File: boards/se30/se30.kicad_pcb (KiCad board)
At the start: 2 copper layers, 116.8 x 59.7 mm, 43 parts, among them J1 Mac SE/30 PDS Interface, J2 Conn_02x05_Odd_Even, U1 ENC624J600-PT, U2 SST39SF010, U3 GAL16V8, U4 GAL16V8, U5 LD1117S33TR_SOT223, Y1 25MHz

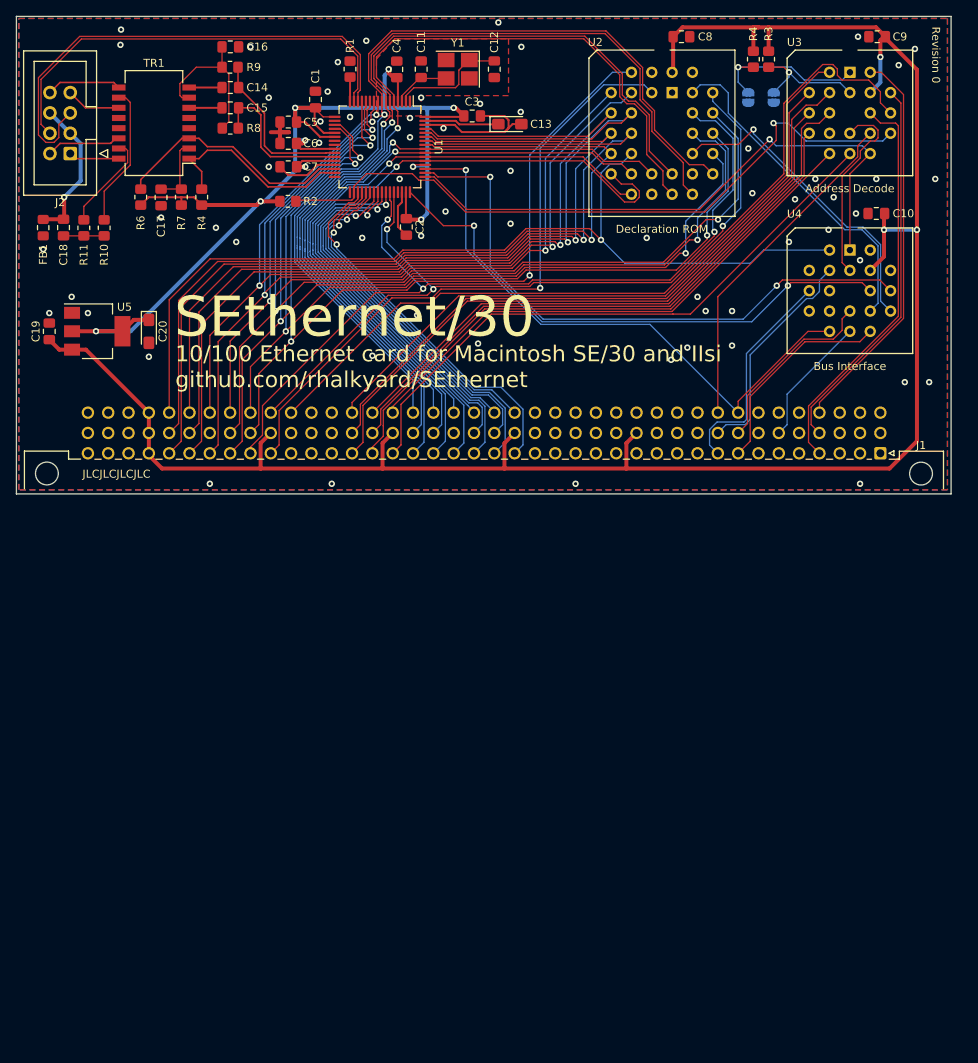
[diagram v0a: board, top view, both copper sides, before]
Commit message: Rev1 hardware
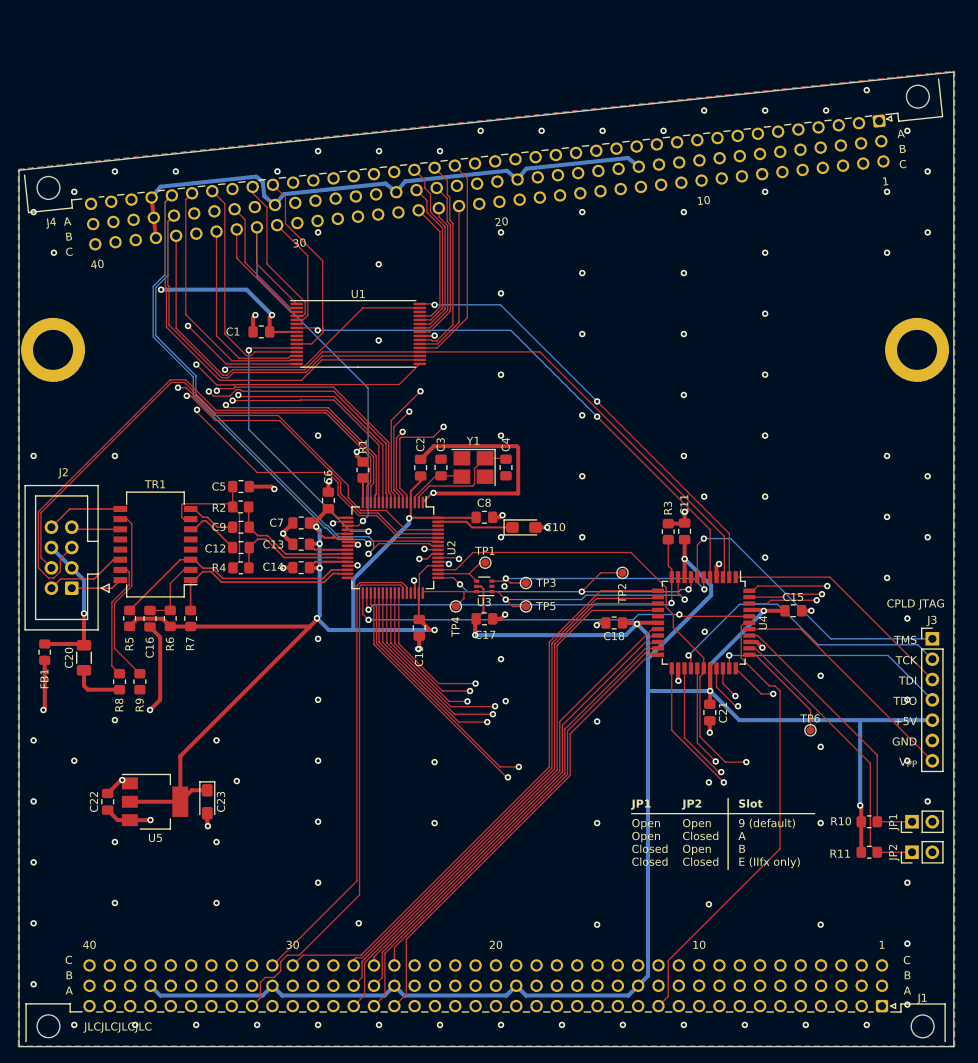
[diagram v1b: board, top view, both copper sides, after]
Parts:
- removed the C10 at (133.5, 49.4)
- removed the R4 at (49.1, 47.4)
- removed the U5 at (36.1, 64.1)
- added C15: 1uF, Capacitor_SMD:C_0805_2012Metric_Pad1.18x1.45mm_HandSolder, F.Cu at (123.1, 99.1)
- added C17: 1uF, Capacitor_SMD:C_0805_2012Metric_Pad1.18x1.45mm_HandSolder, F.Cu at (84.5, 100.1)
- added C18: 1uF, Capacitor_SMD:C_0805_2012Metric_Pad1.18x1.45mm_HandSolder, F.Cu at (100.7, 100.6)
- added C21: 1uF, Capacitor_SMD:C_0805_2012Metric_Pad1.18x1.45mm_HandSolder, F.Cu at (112.7, 111.8)
- added H1: MountingHole, MountingHole:MountingHole_5mm, F.Cu at (30.6, 66.5)
- added H2: MountingHole, MountingHole:MountingHole_5mm, F.Cu at (138.6, 66.5)
- added J3: Conn_01x07, Connector_PinHeader_2.54mm:PinHeader_1x07_P2.54mm_Vertical, F.Cu at (140.5, 102.6)
- added J4: Mac SE/30 PDS Interface, PDS-Ethernet:DIN41612_C_3x40_Female_Horizontal_THT, F.Cu at (35.3, 48.2)
- added R7: 49.9, Resistor_SMD:R_0805_2012Metric_Pad1.20x1.40mm_HandSolder, F.Cu at (47.8, 100.0)
- added TP1: TestPoint, TestPoint:TestPoint_Pad_D1.0mm, F.Cu at (84.6, 93.1)
- added TP2: TestPoint, TestPoint:TestPoint_Pad_D1.0mm, F.Cu at (101.7, 94.3)
- added TP3: TestPoint, TestPoint:TestPoint_Pad_D1.0mm, F.Cu at (89.7, 95.6)
- added TP4: TestPoint, TestPoint:TestPoint_Pad_D1.0mm, F.Cu at (80.9, 98.5)
- added TP5: TestPoint, TestPoint:TestPoint_Pad_D1.0mm, F.Cu at (89.7, 98.5)
- added TP6: TestPoint, TestPoint:TestPoint_Pad_D1.0mm, F.Cu at (125.2, 114.0)
- added U3: 74LVC2G17, Package_TO_SOT_SMD:SOT-363_SC-70-6, F.Cu at (84.5, 96.0)
- C20: renamed from C18; footprint Capacitor_SMD:C_0805_2012Metric_Pad1.18x1.45mm_HandSolder -> Capacitor_SMD:C_1206_3216Metric_Pad1.33x1.80mm_HandSolder
- JP1: renamed from JP2; footprint Jumper:SolderJumper-2_P1.3mm_Open_RoundedPad1.0x1.5mm -> Connector_PinHeader_2.54mm:PinHeader_1x02_P2.54mm_Vertical; moved to F.Cu
- JP2: renamed from JP1; footprint Jumper:SolderJumper-2_P1.3mm_Open_RoundedPad1.0x1.5mm -> Connector_PinHeader_2.54mm:PinHeader_1x02_P2.54mm_Vertical; moved to F.Cu
- U1: renamed from U2; footprint Package_LCC:PLCC-32_THT-Socket -> Package_SO:TSOP-I-32_14.4x8mm_P0.5mm
- U4: renamed from U3; value GAL16V8 -> ATF1502AS-xAx44; footprint Package_LCC:PLCC-20_THT-Socket -> Package_QFP:TQFP-44_10x10mm_P0.8mm
- U5: renamed from U4; value GAL16V8 -> LD1117S33TR_SOT223; footprint Package_LCC:PLCC-20_THT-Socket -> Package_TO_SOT_SMD:SOT-223-3_TabPin2
- moved U5 110.9 mm to (43.3, 122.9)
- moved R11 99.9 mm to (132.6, 129.2), turned to 0 degrees
- moved R10 96.4 mm to (132.6, 125.4), turned to 0 degrees
- moved JP2 95.9 mm to (137.9, 129.2)
- moved JP1 92.8 mm to (137.9, 125.4)
- moved C1 85.4 mm to (56.6, 64.2)
- moved U4 71.2 mm to (111.9, 100.6), turned to -90 degrees
- moved J1 69.1 mm to (134.2, 148.5)
- moved R3 63.0 mm to (107.5, 89.2), turned to -90 degrees
- moved C11 61.8 mm to (109.5, 89.1), turned to 90 degrees
- moved C23 59.3 mm to (49.8, 122.9)
- moved C22 59.3 mm to (37.4, 122.9)
- moved R9 56.9 mm to (41.4, 107.9)
- moved R8 56.9 mm to (38.9, 107.9)
- moved R2 55.0 mm to (54.0, 86.1)
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- renumbered C9 to C1, C13 to C10, C8 to C11, C15 to C12, C6 to C13, C7 to C14, C17 to C16, C2 to C19, C4 to C2, C19 to C22, C20 to C23, C11 to C3, C12 to C4, C16 to C5, C1 to C6, C5 to C7, C3 to C8, C14 to C9, R4 to R10, R3 to R11, R9 to R2, R2 to R3, R8 to R4, R6 to R5, R7 to R6, R11 to R8, R10 to R9, U1 to U2
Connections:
- JP1 pad 1: GND -> /~{SLOTID_1}
- JP1 pad 2: Net-(JP2-B) -> GND
- JP2 pad 1: GND -> /~{SLOTID_0}
- JP2 pad 2: Net-(JP1-B) -> GND
- R10 pad 2: Net-(JP2-B) -> /~{SLOTID_1}
- R11 pad 2: Net-(JP1-B) -> /~{SLOTID_0}
- R3 pad 1: +3.3V -> GND
- U1 pad 1: GND -> A11
- U1 pad 10: A2 -> GND
- U1 pad 11: A1 -> A15
- U1 pad 12: A0 -> A12
- U1 pad 13: D24 -> A7
- U1 pad 14: D25 -> A6
- U1 pad 15: D26 -> A5
- U1 pad 16: GND -> A4
- U1 pad 17: D27 -> A3
- U1 pad 18: D28 -> A2
- U1 pad 19: D29 -> A1
- U1 pad 2: GND -> A9
- U1 pad 20: D30 -> A0
- U1 pad 21: D31 -> D24
- U1 pad 22: GND -> D25
- U1 pad 23: A10 -> D26
- U1 pad 24: /ROM_~{OE} -> GND
- U1 pad 25: A11 -> D27
- U1 pad 26: A9 -> D28
- U1 pad 27: A8 -> D29
- U1 pad 28: A13 -> D30
- U1 pad 29: A14 -> D31
- U1 pad 3: A15 -> A8
- U1 pad 31: /ROM_~{WE} -> A10
- U1 pad 32: +5V -> /ROM_~{OE}
- U1 pad 4: A12 -> A13
- U1 pad 5: A7 -> A14
- U1 pad 6: A6 -> GND
- U1 pad 7: A5 -> /ROM_~{WE}
- U1 pad 8: A4 -> +5V
- U1 pad 9: A3 -> GND
- U2 pad 33: unconnected-(U1-CLKOUT-Pad33) -> /ENC_CLK
- U2 pad 48: /B1SEL -> /B1SEL'
- U2 pad 50: /B0SEL -> /B0SEL'
- U4 pad 1: Net-(JP2-B) -> /TDI
- U4 pad 10: GND -> /B1SEL
- U4 pad 11: A31 -> /ETH_~{INT}
- U4 pad 12: /ROM_~{CS} -> A16
- U4 pad 13: /ETH_CS -> A24
- U4 pad 14: /ETH_~{INT} -> A25
- U4 pad 15: ~{AS} -> A26
- U4 pad 16: A16 -> GND
- U4 pad 17: ~{IRQ3} -> +5V
- U4 pad 18: ~{IRQ2} -> A27
- U4 pad 19: ~{IRQ1} -> A28
- U4 pad 2: Net-(JP1-B) -> /ROM_~{OE}
- U4 pad 20: +5V -> A29
- U4 pad 3: A24 -> A0
- U4 pad 4: A25 -> GND
- U4 pad 5: A26 -> /ROM_~{WE}
- U4 pad 6: A27 -> /B0SEL
- U4 pad 7: A28 -> /TMS
- U4 pad 8: A29 -> /ETH_CS
- U4 pad 9: A30 -> +5V
- U5 pad 1: /ETH_CS -> GND
- U5 pad 2: /ROM_~{CS} -> +3.3V
- U5 pad 3: A0 -> +5V
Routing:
- net +5V: track 249.5 -> 447.8 mm, vias 3 -> 9
- net ~{RESET}: track 0.00 -> 165.7 mm
- net -12V: track 0.00 -> 114.7 mm
- net /PDS Interface/RESV_A1: track 0.00 -> 112.2 mm
- net A2: track 116.4 -> 228.4 mm
- net CPUCLK: track 0.00 -> 111.9 mm
- net A1: track 108.2 -> 219.9 mm
- net /PDS Interface/RESV_A2: track 0.00 -> 111.2 mm
- net /PDS Interface/~{BUSLOCK}: track 0.00 -> 111.1 mm
- net /PDS Interface/~{IPL2}: track 0.00 -> 110.6 mm
- net /PDS Interface/~{CIOUT}: track 0.00 -> 110.5 mm
- net /PDS Interface/~{STERM}: track 0.00 -> 110.1 mm
- net /PDS Interface/~{BGACK}: track 0.00 -> 109.7 mm
- net /PDS Interface/FC2: track 0.00 -> 109.3 mm
- net -5V: track 0.00 -> 109.3 mm
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- added copper zone on In1.Cu, net GND
- added copper zone on In2.Cu, net GND
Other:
- board size 116.8 x 59.7 mm -> 116.8 x 121.8 mm
- copper layers 2 -> 4
- board text added: "+5V"
- board text added: "10/100 Ethernet for Macintosh SE/30 github.com/rhalkyard/SEthernet Revision 1"
- board text added: "9 (default) A B E (IIfx only)"
- board text added: "Build info:"
- board text added: "CPLD JTAG"
- board text added: "GND"
- board text added: "TCK"
- board text added: "TDI"
- board text added: "TDO"
- board text added: "TMS"
- board text added: "V_{PP}"
- board text removed: "10/100 Ethernet card for Macintosh SE/30 and IIsi github.com/rhalkyard/SEthernet"
- board text removed: "9 E A B"
- board text removed: "Address Decode"
- board text removed: "Bus Interface"
- board text removed: "Declaration ROM"
- board text removed: "Revision 0"
